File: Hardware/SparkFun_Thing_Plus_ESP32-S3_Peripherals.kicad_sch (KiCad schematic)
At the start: 31 parts, among them J2 microSD_Friction, J3 JST_2mm_LiPo, J5 Qwiic_RA, U1 RT9080-3.3, U4 MAX17048, U5 MCP73831

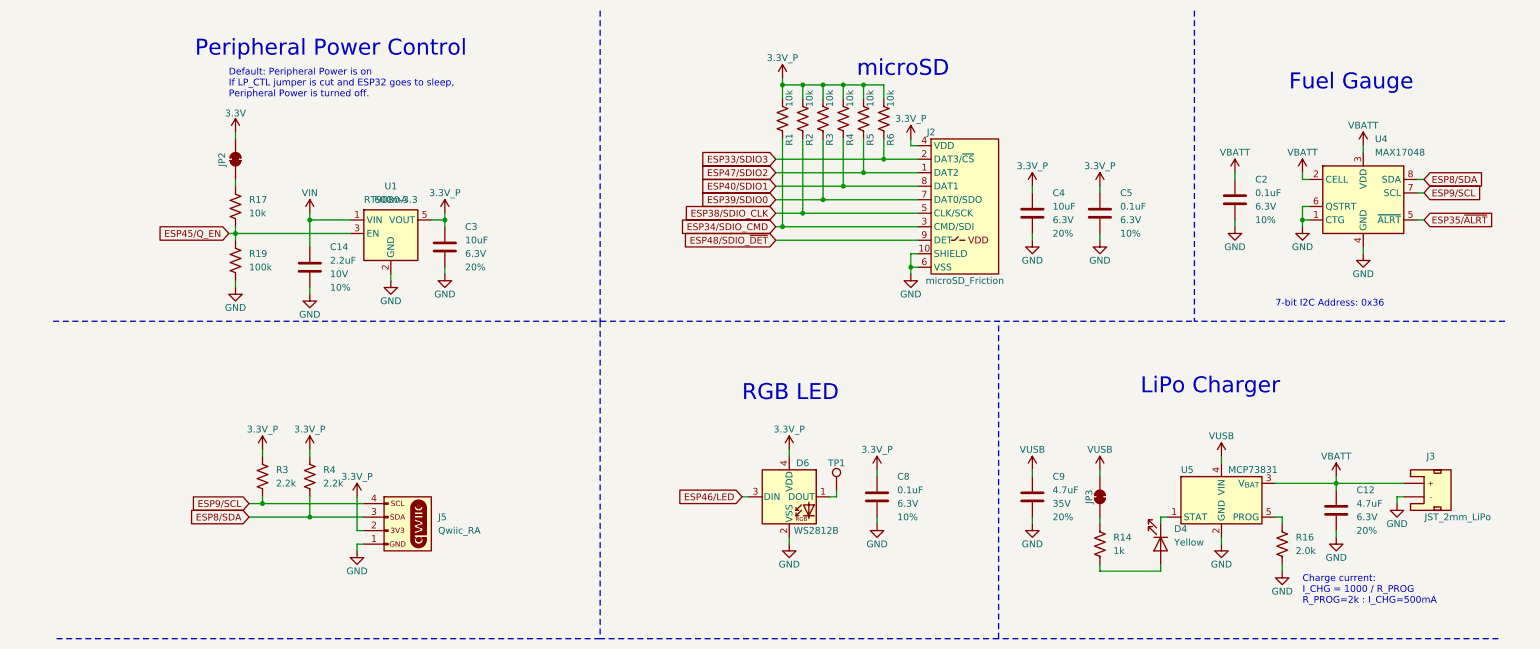
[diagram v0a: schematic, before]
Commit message: initial change to riichi pcb
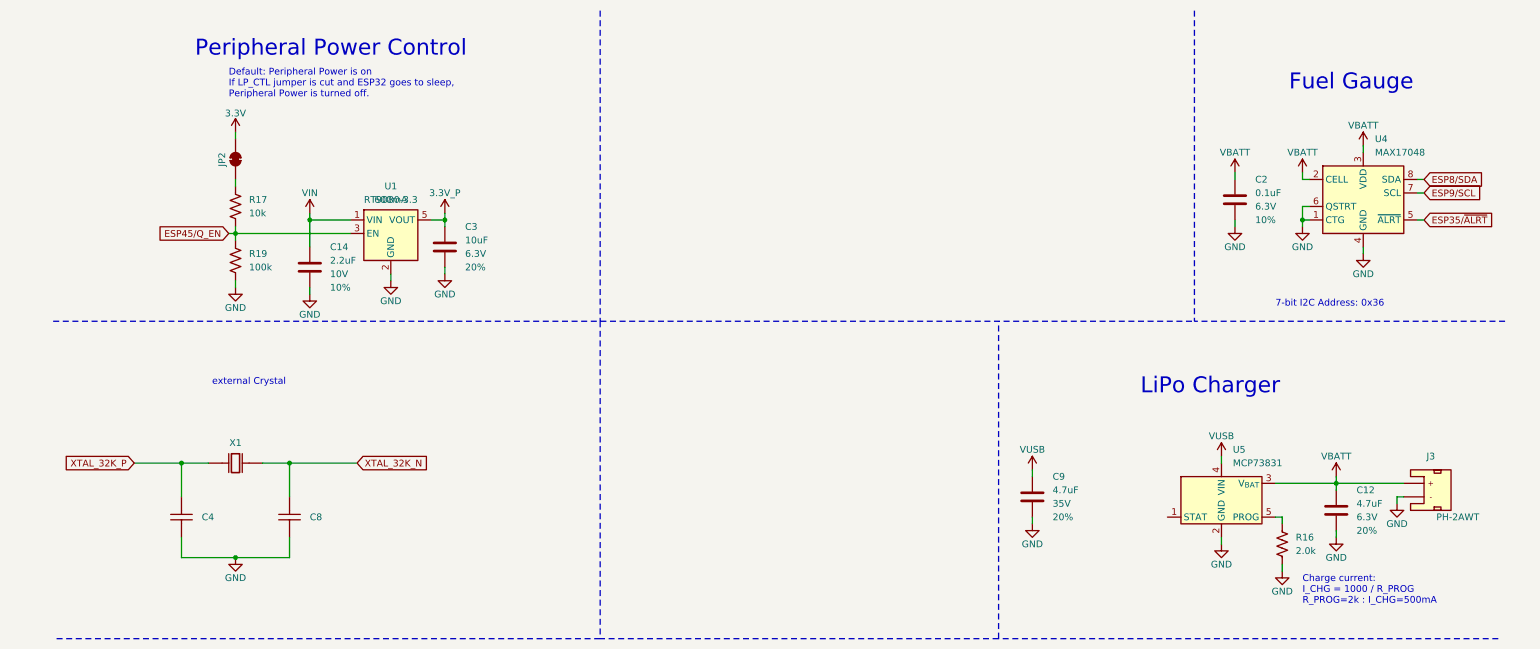
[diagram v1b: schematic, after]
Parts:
- removed C4: 10uF, SparkFun-Capacitor:C_0402_1005Metric, symbol SparkFun-Capacitor:10uF_0402_6.3V_20%
- removed C5, C8: 0.1uF, SparkFun-Capacitor:C_0402_1005Metric, symbol SparkFun-Capacitor:0.1uF_0402_6.3V_10%
- removed D4: Yellow, SparkFun-LED:LED_0603_1608Metric_Yellow, symbol SparkFun-LED:LED_Yellow_0603
- removed D6: WS2812B, SparkFun-LED:WS2812_2020, symbol SparkFun-LED:WS2812B_2020
- removed J2: microSD_Friction, SparkFun-Connector:microSD_Friction_Fit_Common, symbol SparkFun-Connector:microSD_Friction
- removed J5: Qwiic_RA, SparkFun-Connector:JST_SMD_1.0mm-4_RA, symbol SparkFun-Connector:Qwiic_Right_Angle
- removed JP3: ~, SparkFun-Jumper:Jumper_2_NC_Trace, symbol SparkFun-Jumper:SolderJumper_2_Bridged
- removed R1, R2, R3, R4, R5, R6: 10k, SparkFun-Resistor:R_0402_1005Metric, symbol SparkFun-Resistor:10k_0402
- removed R14: 1k, SparkFun-Resistor:R_0402_1005Metric, symbol SparkFun-Resistor:1k_0402
- removed R3, R4: 2.2k, SparkFun-Resistor:R_0402_1005Metric, symbol SparkFun-Resistor:2.2k_0402
- removed TP1: 1.0mm, SparkFun-Connector:TestPoint-1.0mm, symbol SparkFun-Connector:TestPoint_1.0mm
- added C4, C8: 4pF, EasyEDA_Lib:C0402, symbol EasyEDA_Lib:0402CG4R0C500NT
- added X1: 32.768kHz, EasyEDA_Lib:CRYSTAL-SMD_L7.0-W3.2-LS7.5, symbol EasyEDA_Lib:3437S-32.768DT07LLL
- J3: value JST_2mm_LiPo -> PH-2AWT; footprint SparkFun-Connector:JST_SMD_2.0mm-2 -> EasyEDA_Lib:CONN-SMD_PH-2AWT; JLC (none) -> C2763693
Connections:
- net GND: now also C4.1, C8.1
- new net XTAL_32K_N: C8.2, X1.2 (OSC2)
- new net XTAL_32K_P: C4.2, X1.1 (OSC1)
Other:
- note added: "external Crystal"
- note removed: "RGB LED"
- note removed: "microSD"

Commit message: funktioniert wahrscheinlich erst mal
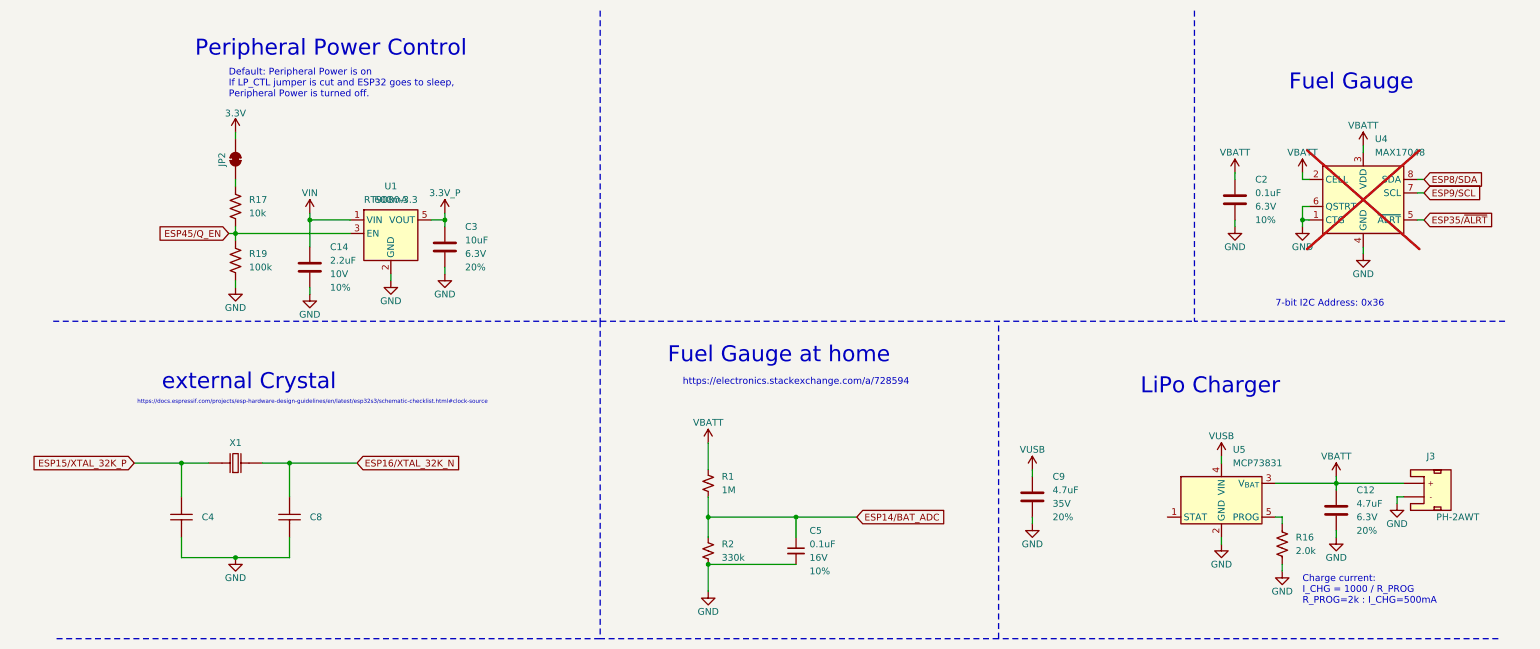
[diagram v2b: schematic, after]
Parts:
- added C5: 0.1uF, PCM_SparkFun-Capacitor:C_0402_1005Metric, symbol PCM_SparkFun-Capacitor:0.1uF_0402_16V_10%
- added R1: 1M, PCM_SparkFun-Resistor:R_0603_1608Metric, symbol PCM_SparkFun-Resistor:1M_0603
- added R2: 330k, PCM_SparkFun-Resistor:R_0603_1608Metric, symbol PCM_SparkFun-Resistor:330_0603
- C4, C8: value 4pF -> 15pF
- U4: now not fitted
- X1: footprint EasyEDA_Lib:CRYSTAL-SMD_L7.0-W3.2-LS7.5 -> EasyEDA_Lib:FC-135R_L3.2-W1.5; symbol EasyEDA_Lib:3437S-32.768DT07LLL -> EasyEDA_Lib:Q13FC1350000400; LCSC Part Name 32.768kHz ±20ppm 7pF -> 32.768kHz ±20ppm 12.5pF; Manufacturer HCI(杭晶) -> EPSON(爱普生); Manufacturer Part 3437S-32.768DT07LLL -> Q13FC13500004; Supplier Part C20624187 -> C32346
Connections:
- net GND: now also C5.2, R2.1
- net VBATT: now also R1.2
- net XTAL_32K_N renamed ESP16/XTAL_32K_N
- net XTAL_32K_P renamed ESP15/XTAL_32K_P
- new net ESP14/BAT_ADC: C5.1, R1.1, R2.2
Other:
- note added: "Fuel Gauge at home"
- note added: "https://docs.espressif.com/projects/esp-hardware-design-guidelines/en/latest/esp32s3/schematic-checklist.html#clock-source"
- note added: "https://electronics.stackexchange.com/a/728594"

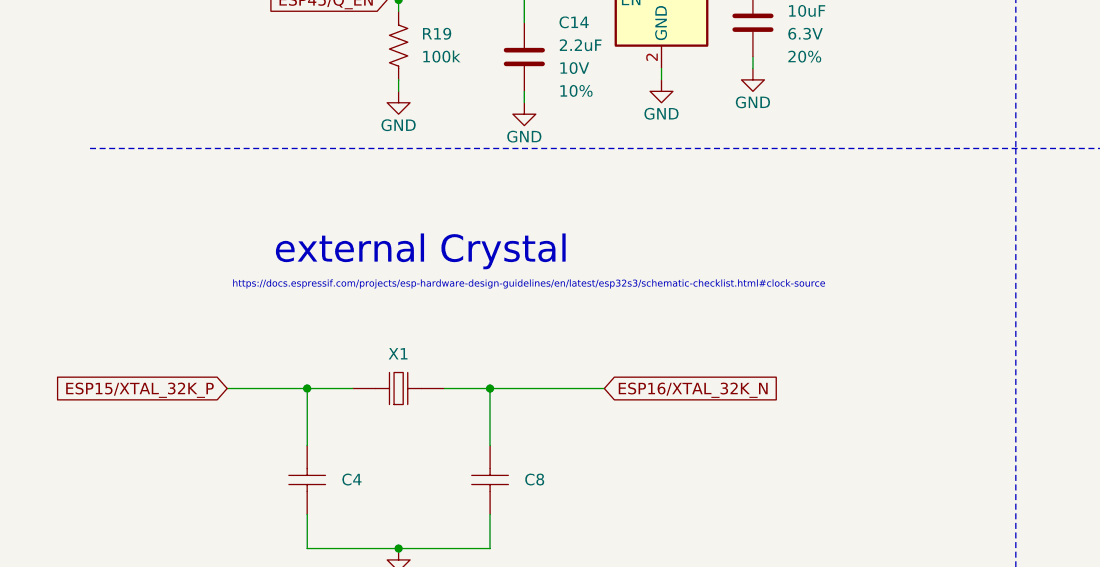
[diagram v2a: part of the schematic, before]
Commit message: add link
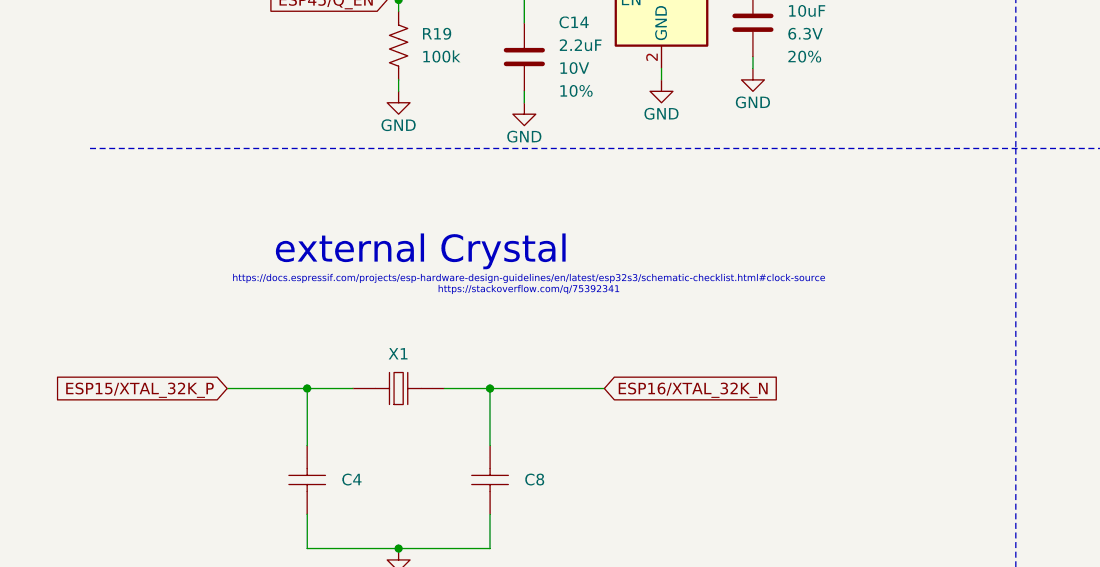
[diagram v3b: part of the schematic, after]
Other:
- note added: "https://docs.espressif.com/projects/esp-hardware-design-guidelines/en/latest/esp32s3/schematic-checklist.html#clock-source https://stackoverflow.com/q/75392341"
- note removed: "https://docs.espressif.com/projects/esp-hardware-design-guidelines/en/latest/esp32s3/schematic-checklist.html#clock-source"
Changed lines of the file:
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@@
 	(generator_version "9.0")
 	(paper "A4")
-	(text "https://docs.espressif.com/projects/esp-hardware-design-guidelines/en/latest/esp32s3/schematic-checklist.html#clock-source"
+	(text "https://docs.espressif.com/projects/esp-hardware-design-guidelines/en/latest/esp32s3/schematic-checklist.html#clock-source\nhttps://stackoverflow.com/q/75392341"
 		(exclude_from_sim no)
 		(at 61.468 86.36 0)
